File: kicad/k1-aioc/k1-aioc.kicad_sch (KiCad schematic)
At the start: 55 parts, among them J1 12401832E402A, J2 Conn_01x07_Male, Q1 PZT2222A, U1 TLV1117LV-33, U2 STM32F373CBTx, U3 TLV1117LV-33, U4 CRE1S0505SC, U5 ADUM3160, Y1 8MHz/20pF

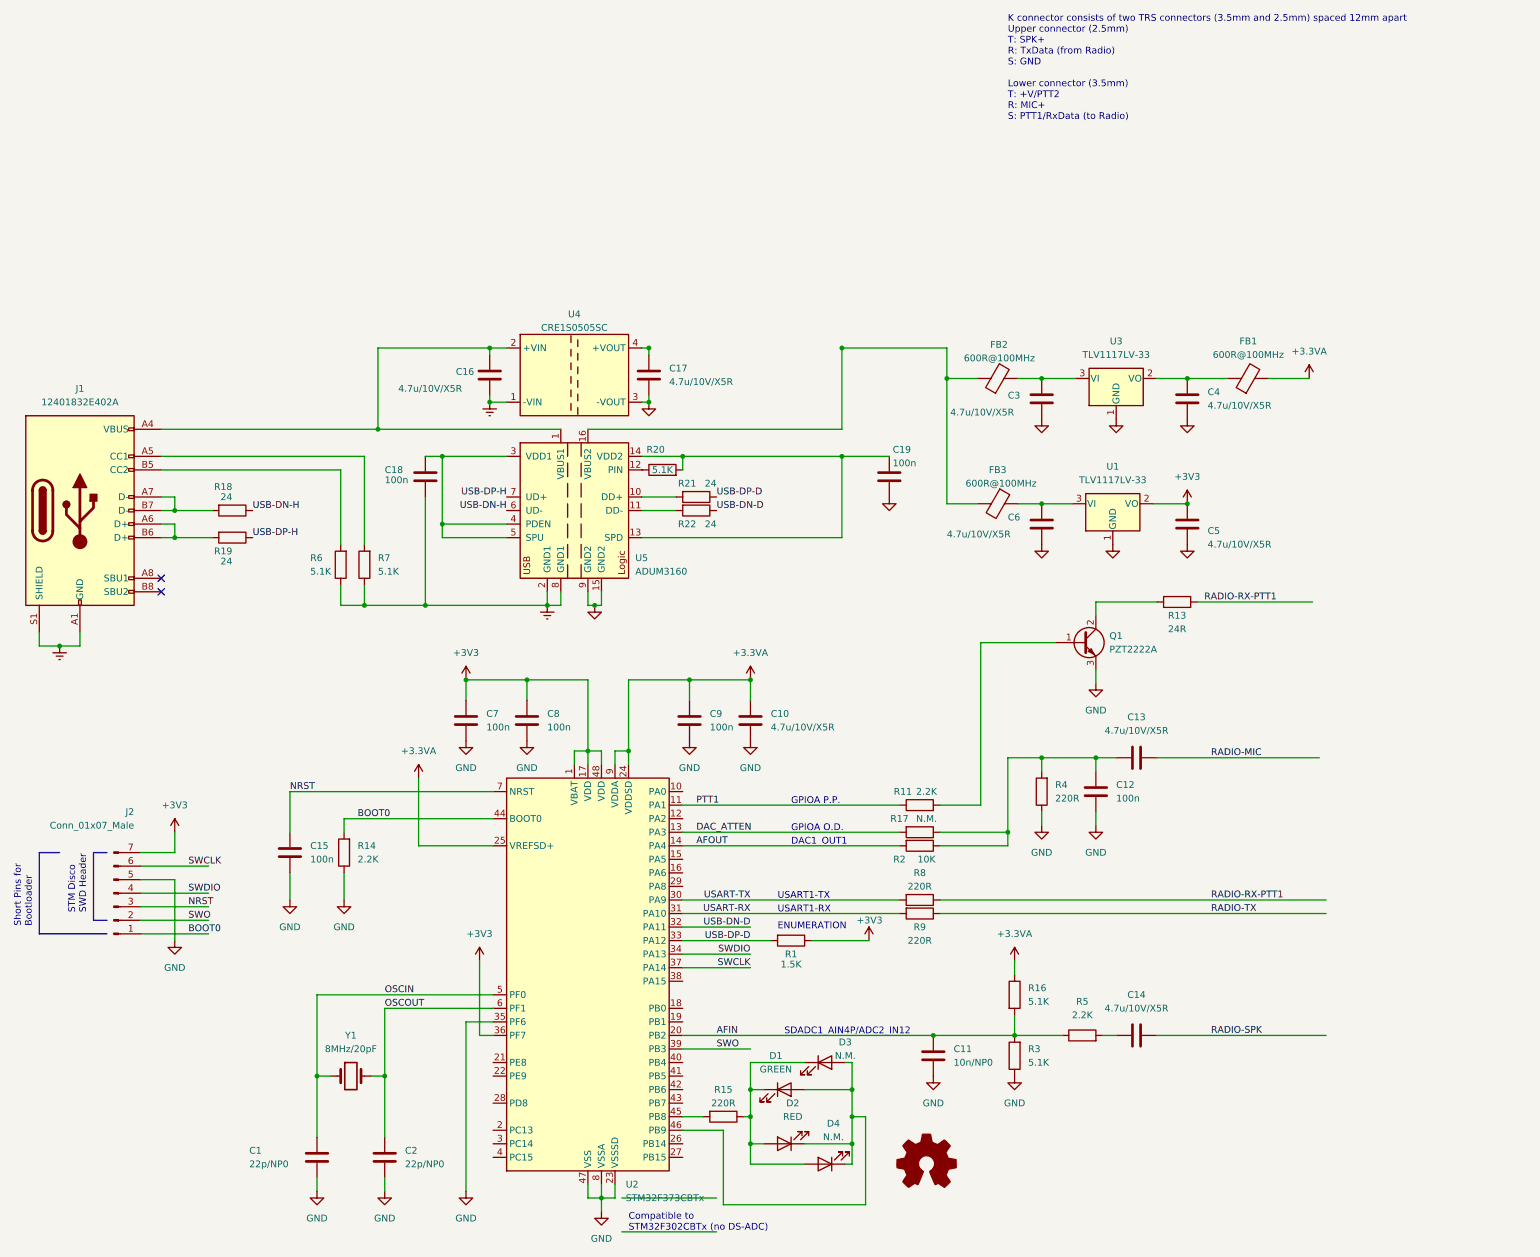
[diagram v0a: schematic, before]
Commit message: Adding two TRRS jacks for I/O (digirig pinout)
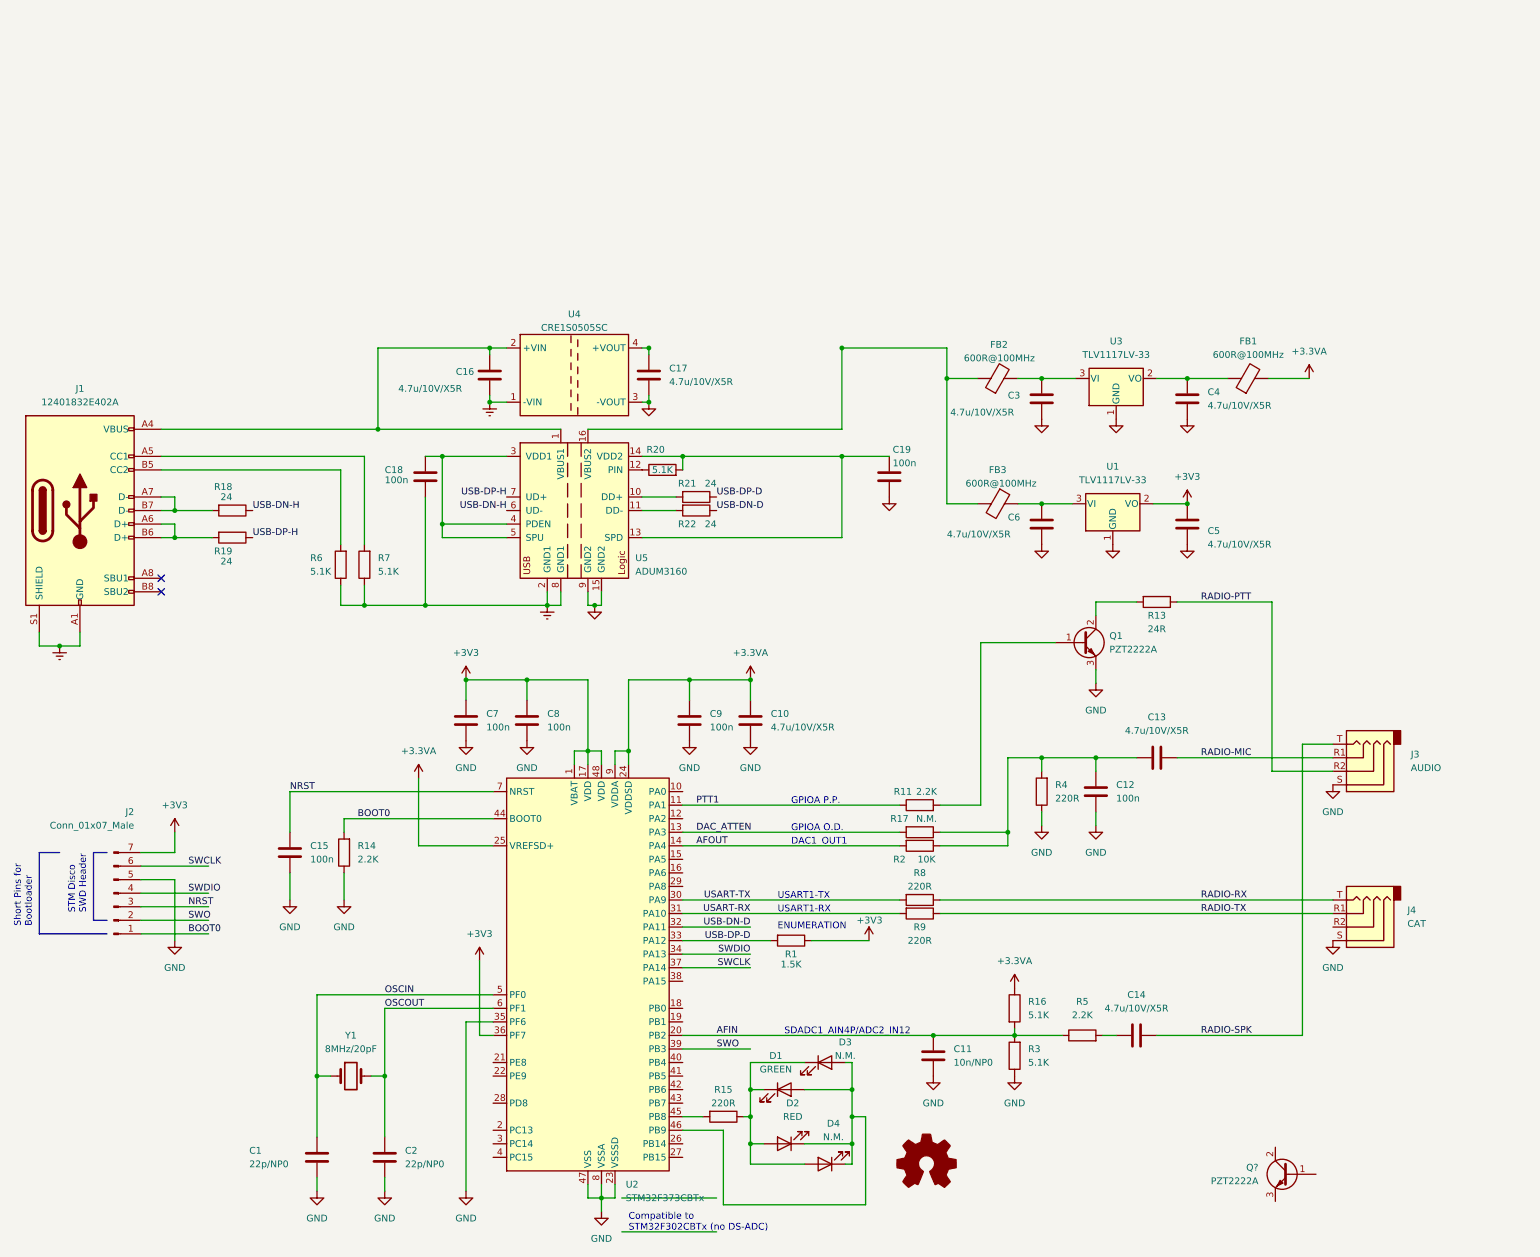
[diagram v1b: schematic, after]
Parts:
- added J3: AUDIO, Connector_Audio:Jack_3.5mm_PJ320E_Horizontal, symbol Connector:AudioJack4
- added J4: CAT, Connector_Audio:Jack_3.5mm_PJ320E_Horizontal, symbol Connector:AudioJack4
- added Q?: PZT2222A, Package_TO_SOT_SMD:SOT-223-3_TabPin2, symbol Transistor_BJT:PZT2222A
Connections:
- net GND: now also J3.S, J4.S
- net RADIO-MIC: now also J3.R1
- net RADIO-SPK: now also J3.T
- net RADIO-TX: now also J4.R1
- net RADIO-RX-PTT1 renamed RADIO-PTT
- net RADIO-PTT: now also J3.R2; no longer R8.1
- new net RADIO-RX: J4.T, R8.1
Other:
- note removed: "K connector consists of two TRS connectors (3.5mm and 2.5mm) spaced 12mm apart Upper connector (2.5mm) T: SPK+ R: TxData (from Radio) S: GND Lower connector (3.5mm) T: +V/PTT2 R: MIC+ S: PTT1/RxData (to Radio)"
- moved on the sheet: C13, R13, R16
